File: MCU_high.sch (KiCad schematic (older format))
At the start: 1 part

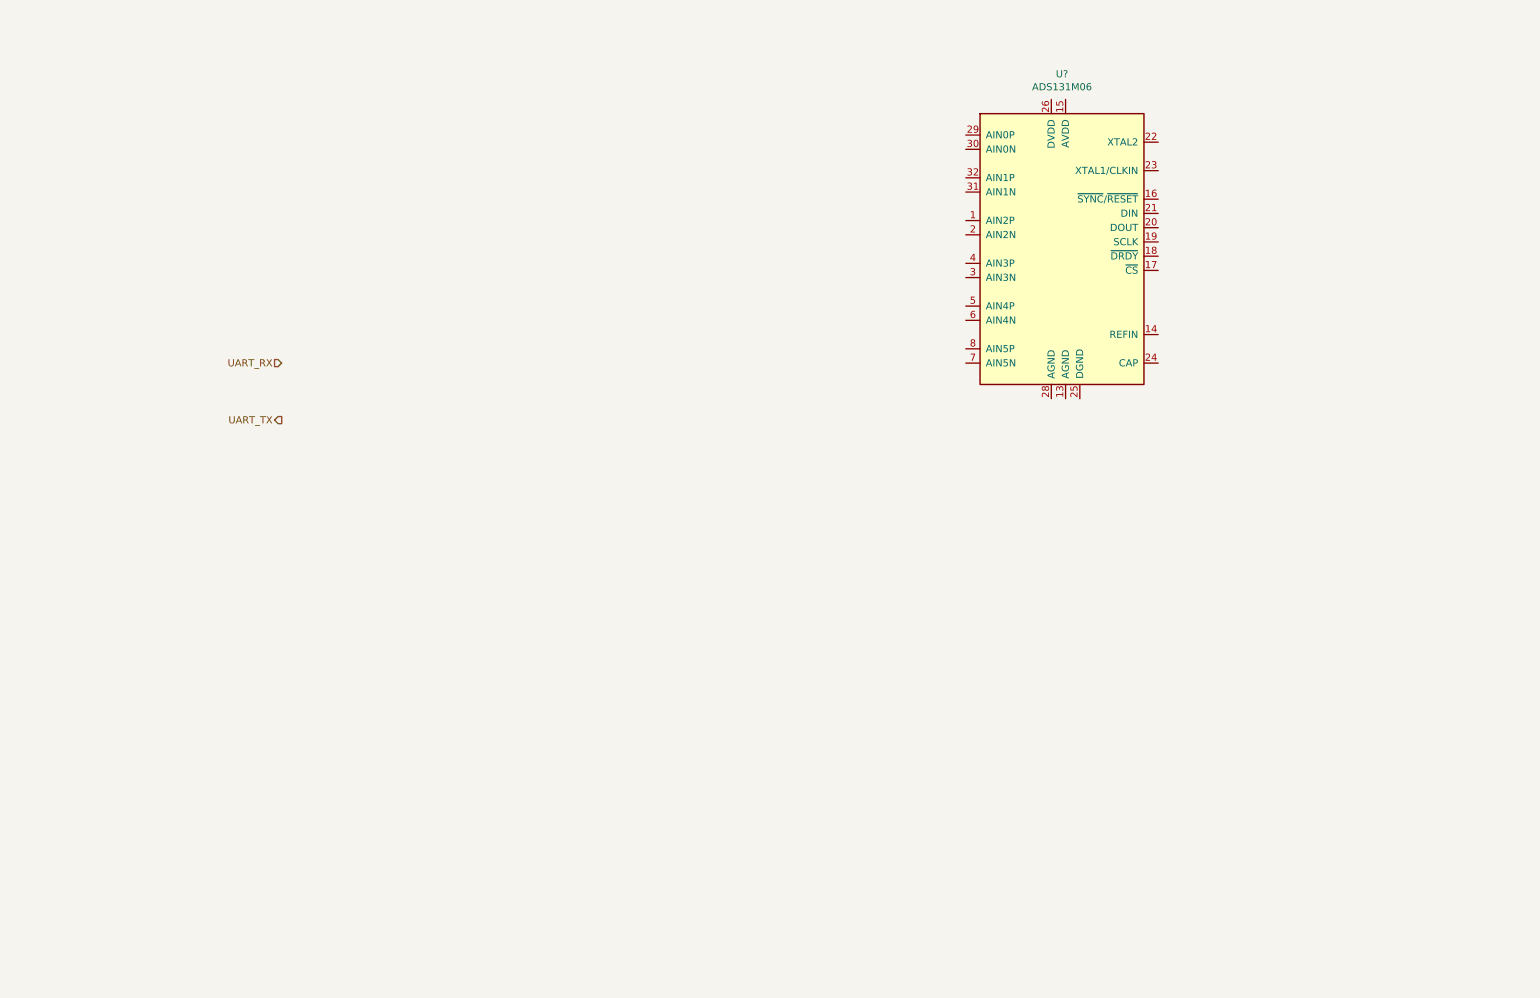
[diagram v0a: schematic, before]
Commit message: - high side (supply, MCU) - low side MCU - much small changes
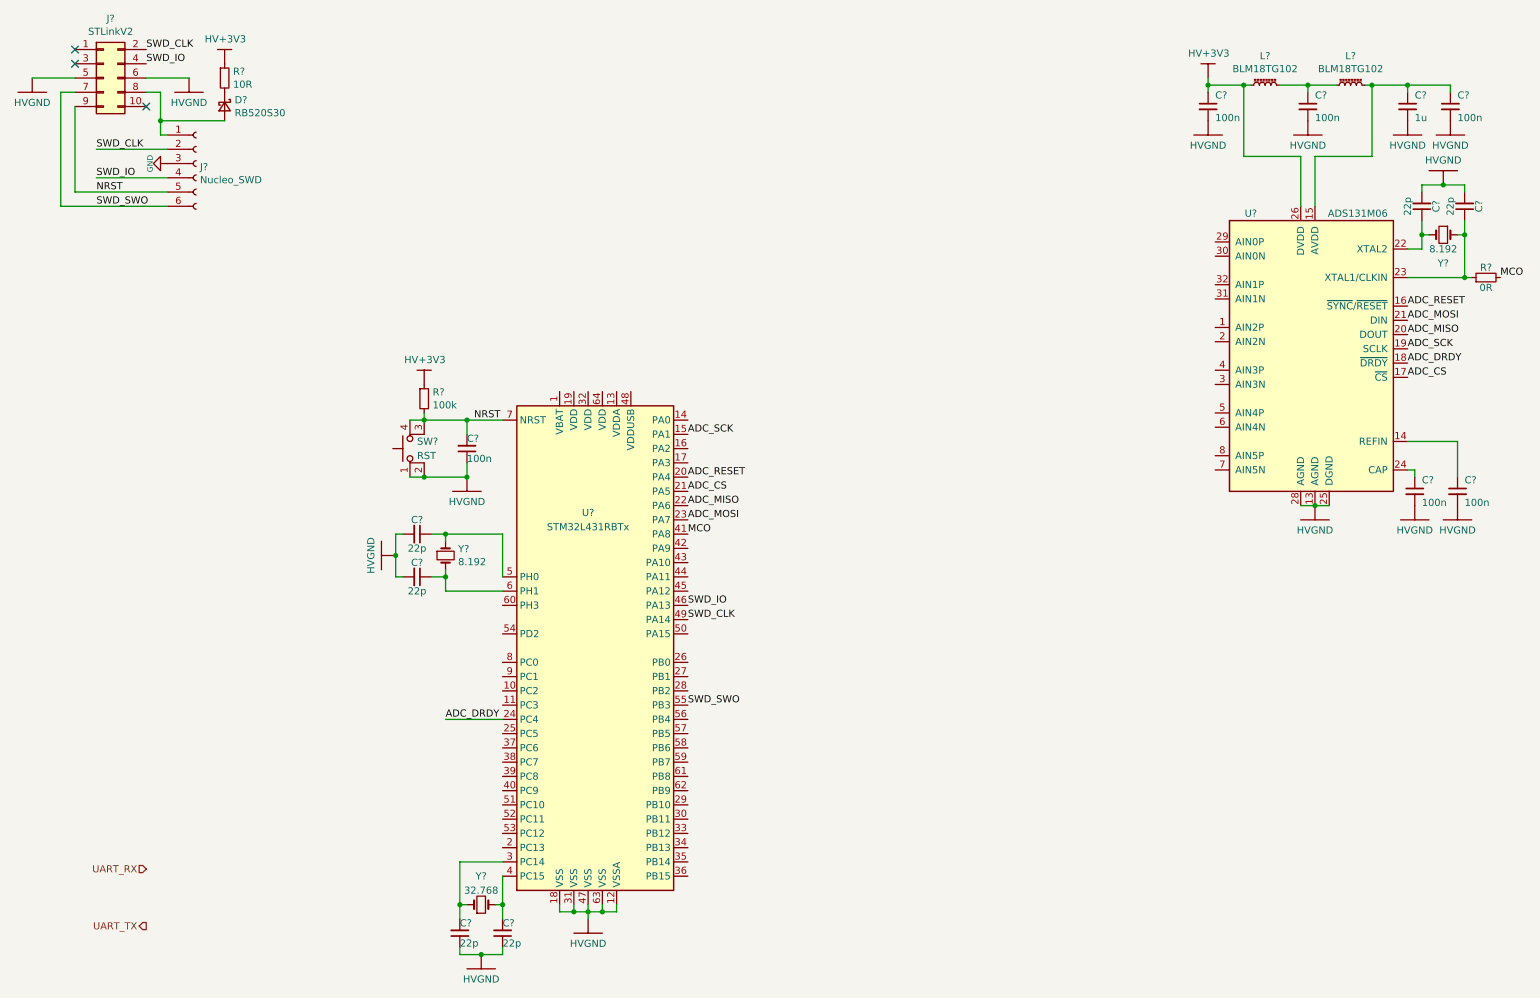
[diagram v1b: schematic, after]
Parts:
- removed U?: ADS131M06, miscellaneous_my:TQFP-32_5x5mm_P0.5mm_edges, symbol miscellaneous:ADS131M06
- added C? (x6): 100n, Capacitor_SMD:C_0603_1608Metric_Pad1.05x0.95mm_HandSolder, symbol Device:C_Small
- added C? (x6): 22p, Capacitor_SMD:C_0603_1608Metric_Pad1.05x0.95mm_HandSolder, symbol Device:C_Small
- added C?: 1u, Capacitor_SMD:C_0603_1608Metric_Pad1.05x0.95mm_HandSolder, symbol Device:C_Small
- added D?: RB520S30, miscellaneous_my:D_SOD-323-523_HandSoldering, symbol Device:D_Schottky_Small
- added J?: STLinkV2, miscellaneous_my:ST-LinkV2_FakeStm8Stm32_vertical, symbol Connector_Generic:Conn_02x05_Odd_Even
- added J?: Nucleo_SWD, Connector_PinSocket_2.54mm:PinSocket_1x06_P2.54mm_Vertical, symbol Connector:Conn_01x06_Female
- added L? (x2): BLM18TG102, Resistor_SMD:R_0603_1608Metric_Pad1.05x0.95mm_HandSolder, symbol Device:L_Core_Ferrite_Small
- added R?: 100k, Resistor_SMD:R_0603_1608Metric_Pad1.05x0.95mm_HandSolder, symbol Device:R_Small
- added R?: 0R, Resistor_SMD:R_0603_1608Metric_Pad1.05x0.95mm_HandSolder, symbol Device:R_Small
- added R?: 10R, Resistor_SMD:R_0603_1608Metric_Pad1.05x0.95mm_HandSolder, symbol Device:R_Small
- added SW?: RST, Button_Switch_SMD:SW_Push_1P1T_NO_6x6mm_H9.5mm, symbol Switch:SW_MEC_5E
- added U?: STM32L431RBTx, Package_QFP:LQFP-64_10x10mm_P0.5mm, symbol MCU_ST_STM32L4:STM32L431RBTx
- added U?: ADS131M06, miscellaneous_my:TQFP-32_5x5mm_P0.5mm_edges, symbol miscellaneous:ADS131M06
- added Y?: 8.192, Crystal:Crystal_HC49-4H_Vertical, symbol Device:Crystal_Small
- added Y?: 32.768, Crystal:Crystal_AT310_D3.0mm_L10.0mm_Horizontal_1EP_style2, symbol Device:Crystal_Small
- added Y?: 8.192, Crystal:Crystal_AT310_D3.0mm_L10.0mm_Horizontal_1EP_style2, symbol Device:Crystal_Small
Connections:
- new net: C?.2, U?.3 (PC14), Y?.1
- new net: C?.2, U?.4 (PC15), Y?.2
- new net: C?.1, U?.5 (PH0), Y?.1
- new net: C?.1, U?.6 (PH1), Y?.2
- new net: C?.1, U?.14 (REFIN)
- new net: C?.1, C?.1, L?.2, U?.15 (AVDD)
- new net: C?.1, U?.22 (XTAL2), Y?.2
- new net: C?.1, R?.1, U?.23 (XTAL1/CLKIN), Y?.1
- new net: C?.1, U?.24 (CAP)
- new net: C?.1, L?.1, L?.2
- new net: D?.2 (A), J?.1 (Pin_1), J?.8 (Pin_8)
- new net: D?.1 (K), R?.2
- new net ADC_CS: U?.17 (~CS), U?.21 (PA5)
- new net ADC_DRDY: U?.18 (~DRDY), U?.24 (PC4)
- new net ADC_MISO: U?.20 (DOUT), U?.22 (PA6)
- new net ADC_MOSI: U?.21 (DIN), U?.23 (PA7)
- new net ADC_RESET: U?.16 (~SYNC~/~RESET), U?.20 (PA4)
- new net ADC_SCK: U?.15 (PA1), U?.19 (SCLK)
- new net GND: J?.3 (Pin_3)
- new net HV+3V3: C?.1, L?.1, R?.1, R?.1, U?.26 (DVDD)
- new net HVGND: C?.1, C?.1, C?.1, C?.2, C?.2, C?.2, C?.2, C?.2, C?.2, C?.2, C?.2, C?.2, C?.2, J?.5 (Pin_5), J?.6 (Pin_6), SW?.1, SW?.2, U?.12 (VSSA), U?.13 (AGND), U?.18 (VSS), U?.25 (DGND), U?.28 (AGND), U?.31 (VSS), U?.47 (VSS), U?.63 (VSS)
- new net MCO: R?.2, U?.41 (PA8)
- new net NRST: C?.2, J?.5 (Pin_5), J?.9 (Pin_9), R?.2, SW?.3 (K), SW?.4 (A), U?.7 (NRST)
- new net SWD_CLK: J?.2 (Pin_2), J?.2 (Pin_2), U?.49 (PA14)
- new net SWD_IO: J?.4 (Pin_4), J?.4 (Pin_4), U?.46 (PA13)
- new net SWD_SWO: J?.6 (Pin_6), J?.7 (Pin_7), U?.55 (PB3)
- no-connect marks 0 -> 3
